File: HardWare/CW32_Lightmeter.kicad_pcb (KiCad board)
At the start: 2 copper layers, 35 x 37.3 mm, 50 parts, among them J1 USB_C_Receptacle, J2 Conn_01x04_Pin, SW1 TM-2022-3, SW2 Power_KEY, U1 CW32F030C8T6, U2 CH340C, U3 BH1750FVI-TR, U4 TP4055, U5 EC190707, U6 RT9013-33GB, X1 12MHz

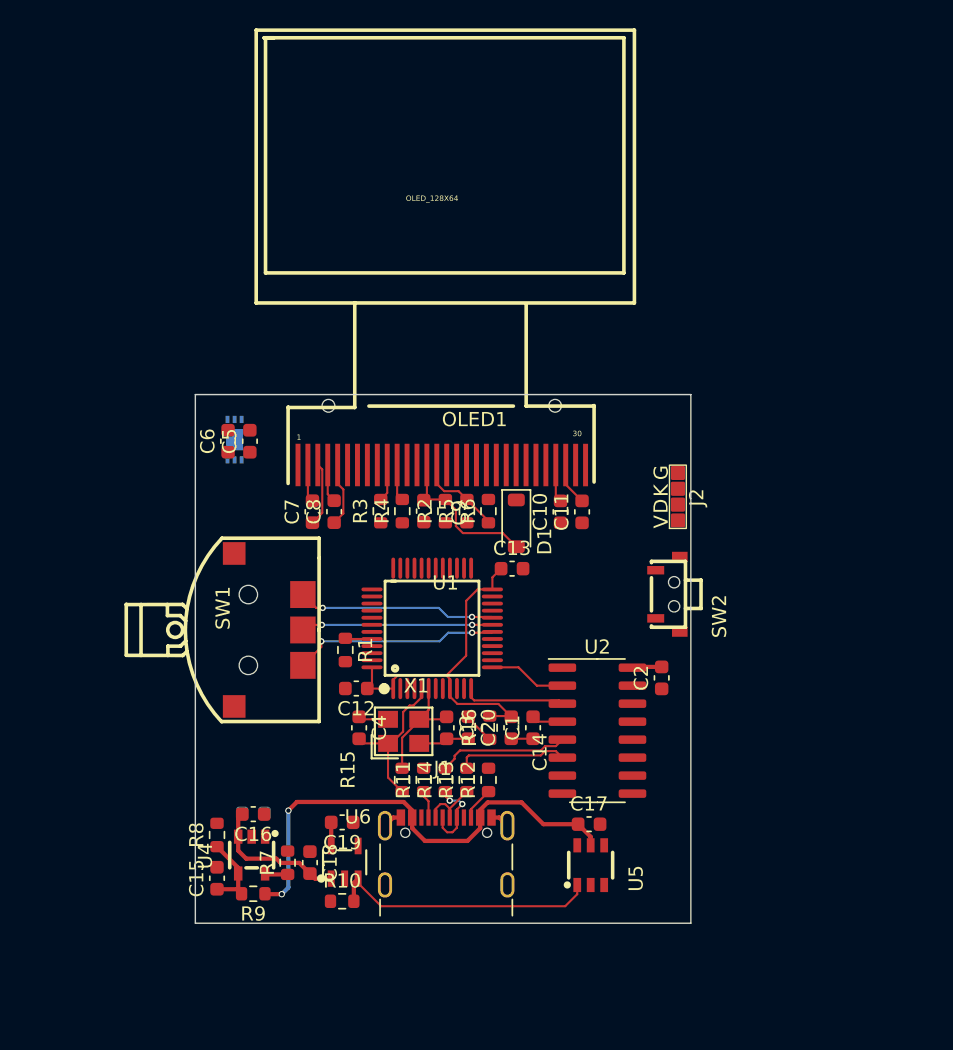
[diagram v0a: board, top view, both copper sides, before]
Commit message: Finished PCB Layout
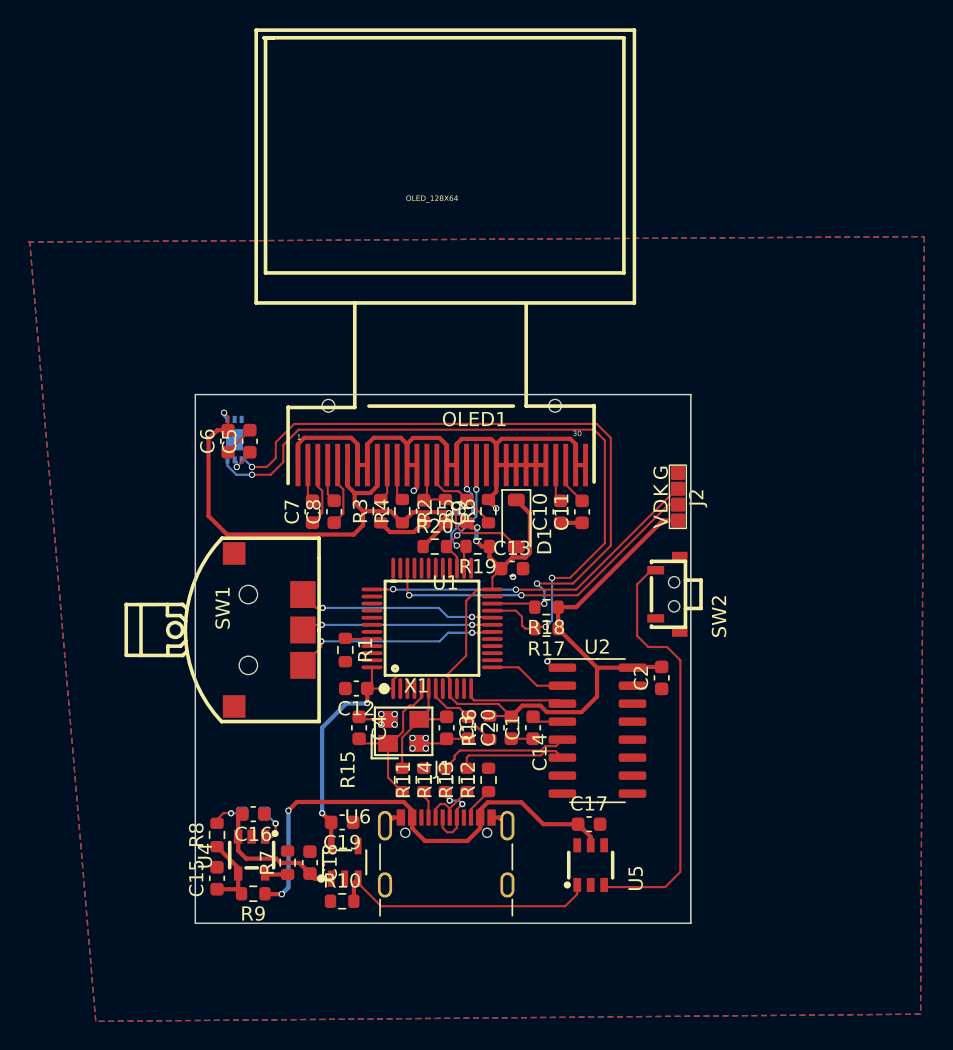
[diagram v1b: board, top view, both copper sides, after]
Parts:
- added R17: 4K7, Resistor_SMD:R_0603_1608Metric, F.Cu at (53.1, 98.9)
- added R18: 4K7, Resistor_SMD:R_0603_1608Metric, F.Cu at (53.1, 97.4)
- added R19: 4K7, Resistor_SMD:R_0603_1608Metric, F.Cu at (48.3, 93.1)
- added R20: 4K7, Resistor_SMD:R_0603_1608Metric, F.Cu at (45.2, 93.1)
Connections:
- U1 pad 26: unconnected-(U1-PB13-Pad26) -> /OLED_SCL
- U1 pad 27: unconnected-(U1-PB14-Pad27) -> /OLED_SDA
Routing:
- net +3.3V: track 29.5 -> 121.4 mm, vias 0 -> 7
- net GND: track 9.97 -> 62.2 mm, vias 0 -> 12
- net /BH1750_SCL: track 0.00 -> 50.0 mm, vias 0 -> 3
- net /BH1750_SDA: track 0.00 -> 48.0 mm, vias 0 -> 3
- net Net-(U5-KEY): track 0.00 -> 29.9 mm
- net /SWCLK: track 0.00 -> 24.6 mm, vias 0 -> 2
- net /SWDIO: track 0.00 -> 23.6 mm, vias 0 -> 2
- net /OLED_SCL: track 0.00 -> 8.89 mm, vias 0 -> 2
- net /OLED_SDA: track 0.00 -> 8.47 mm, vias 0 -> 2
- net /NRST: track 2.23 -> 5.68 mm
- net Net-(D2-K): track 0.00 -> 2.62 mm, vias 0 -> 1
- net Net-(D2-A): track 0.00 -> 2.24 mm, vias 0 -> 1
- net Net-(U3-DVI): track 0.00 -> 2.00 mm, vias 0 -> 1
- added copper zone on B.Cu, net GND
- added copper zone on F.Cu, net GND
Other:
- board text added: "0"
- board text added: "0 mm"
- board text added: "0.01 mm"
- board text added: "0.02"
- board text added: "0.035 mm"
- board text added: "1"
- board text added: "1.51 mm"
- board text added: "3.3"
- board text added: "4.5"
- board text added: "B.Cu"
- board text added: "B.Mask"
- board text added: "B.Paste"
- board text added: "B.Silkscreen"
- board text added: "Bottom Silk Screen"
- board text added: "Bottom Solder Mask"
- board text added: "Bottom Solder Paste"
- board text added: "Epsilon R（相对介电常数）"
- board text added: "F.Cu"
- board text added: "F.Mask"
- board text added: "F.Paste"
- board text added: "F.Silkscreen"
- board text added: "FR4"
- board text added: "Loss Tangent（损耗角正切）"
- board text added: "Not specified"
- board text added: "Top Silk Screen"
- board text added: "Top Solder Mask"
- board text added: "Top Solder Paste"
- board text added: "copper"
- board text added: "core"
- board text added: "层名称"
- board text added: "材料"
- board text added: "电介质"
- board text added: "类型"
- board text added: "线宽 (mm)"
- board text added: "颜色"
